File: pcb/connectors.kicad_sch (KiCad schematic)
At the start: 5 parts, among them J20 DTM1312PA12PBR008, U8 EEC-325X4B

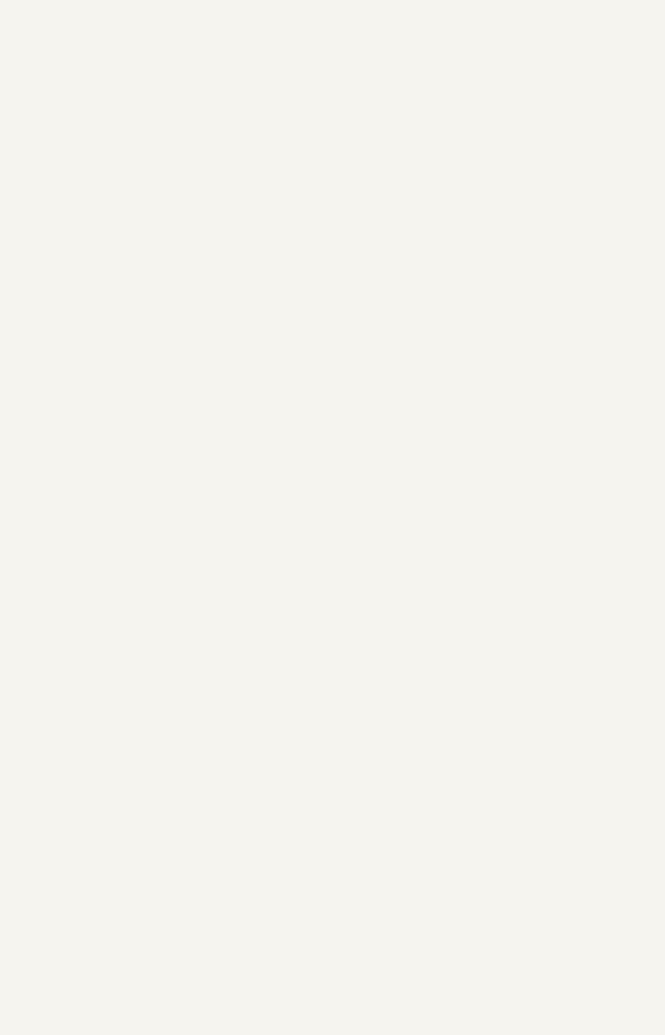
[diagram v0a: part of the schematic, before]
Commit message: added alternative 6-pin headers. Added uart3 test points. V5.2pre2
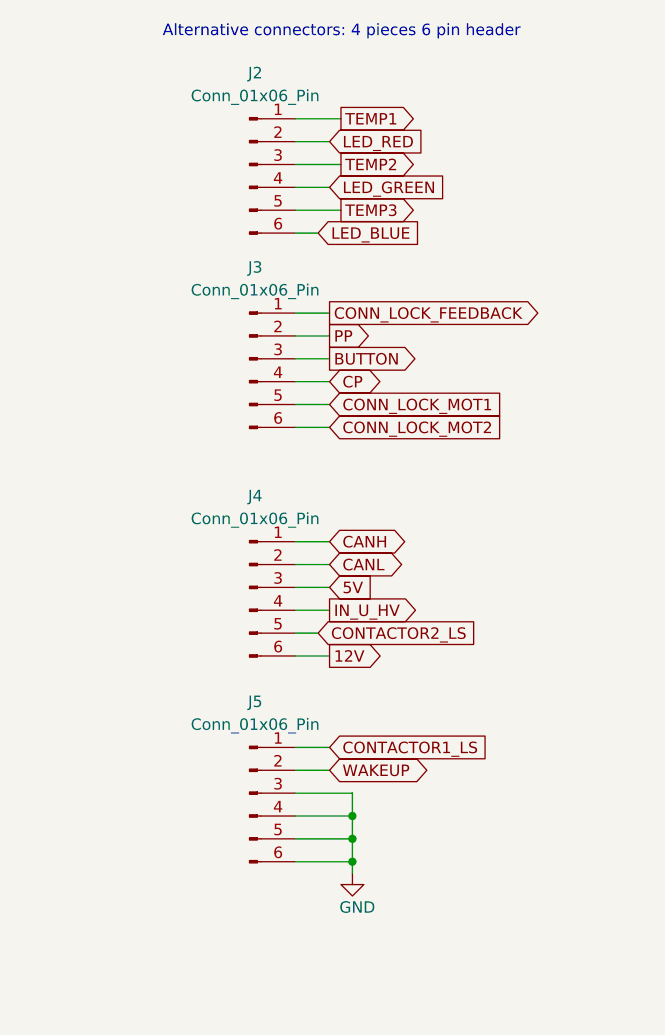
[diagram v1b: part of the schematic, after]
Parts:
- added J2, J3, J4, J5: Conn_01x06_Pin, Connector_PinHeader_2.54mm:PinHeader_1x06_P2.54mm_Vertical, symbol Connector:Conn_01x06_Pin
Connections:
- net 12V: now also J4.6 (Pin_6)
- net 5V: now also J4.3 (Pin_3)
- net BUTTON: now also J3.3 (Pin_3)
- net CANH: now also J4.1 (Pin_1)
- net CANL: now also J4.2 (Pin_2)
- net CONN_LOCK_FEEDBACK: now also J3.1 (Pin_1)
- net CONN_LOCK_MOT1: now also J3.5 (Pin_5)
- net CONN_LOCK_MOT2: now also J3.6 (Pin_6)
- net CONTACTOR1_LS: now also J5.1 (Pin_1)
- net CONTACTOR2_LS: now also J4.5 (Pin_5)
- net CP: now also J3.4 (Pin_4)
- net GND: now also J5.3 (Pin_3), J5.4 (Pin_4), J5.5 (Pin_5), J5.6 (Pin_6)
- net IN_U_HV: now also J4.4 (Pin_4)
- net LED_BLUE: now also J2.6 (Pin_6)
- net LED_GREEN: now also J2.4 (Pin_4)
- net LED_RED: now also J2.2 (Pin_2)
- net PP: now also J3.2 (Pin_2)
- net TEMP1: now also J2.1 (Pin_1)
- net TEMP2: now also J2.3 (Pin_3)
- net TEMP3: now also J2.5 (Pin_5)
- net WAKEUP: now also J5.2 (Pin_2)
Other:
- note added: "Alternative connectors: 4 pieces 6 pin header"
